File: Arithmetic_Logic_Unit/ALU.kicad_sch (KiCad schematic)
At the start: 32 parts, among them U10 74LS245, U11 74LS173, U4 74LS08, U5 74LS86, U6 74LS86, U7 74LS02, U8 74LS283, U9 74LS283

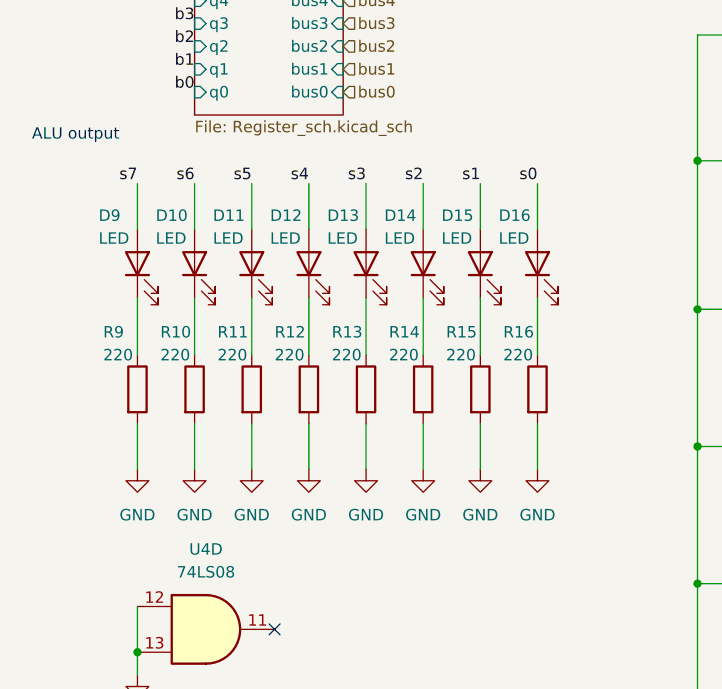
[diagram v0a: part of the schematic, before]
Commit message: layed out PCB
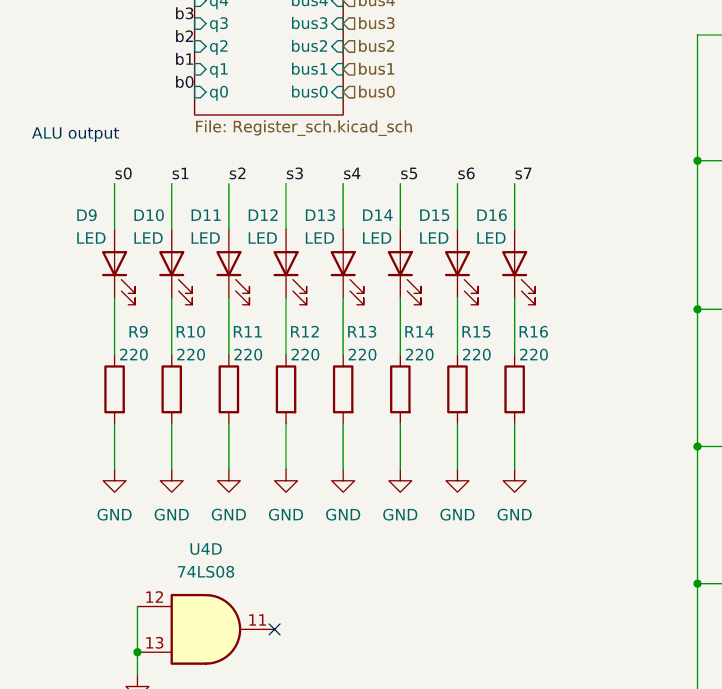
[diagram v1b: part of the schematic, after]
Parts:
- renumbered D15 to D10, D14 to D11, D13 to D12, D12 to D13, D11 to D14, D10 to D15, D9 to D16, D16 to D9, R15 to R10, R14 to R11, R13 to R12, R12 to R13, R11 to R14, R10 to R15, R9 to R16, R16 to R9
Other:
- moved on the sheet: D10, D11, D12, D13, D14, D15, D16, D9, R10, R11, R12, R13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
